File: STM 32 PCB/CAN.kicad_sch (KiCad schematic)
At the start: 6 parts, among them U1 SN65HVD230

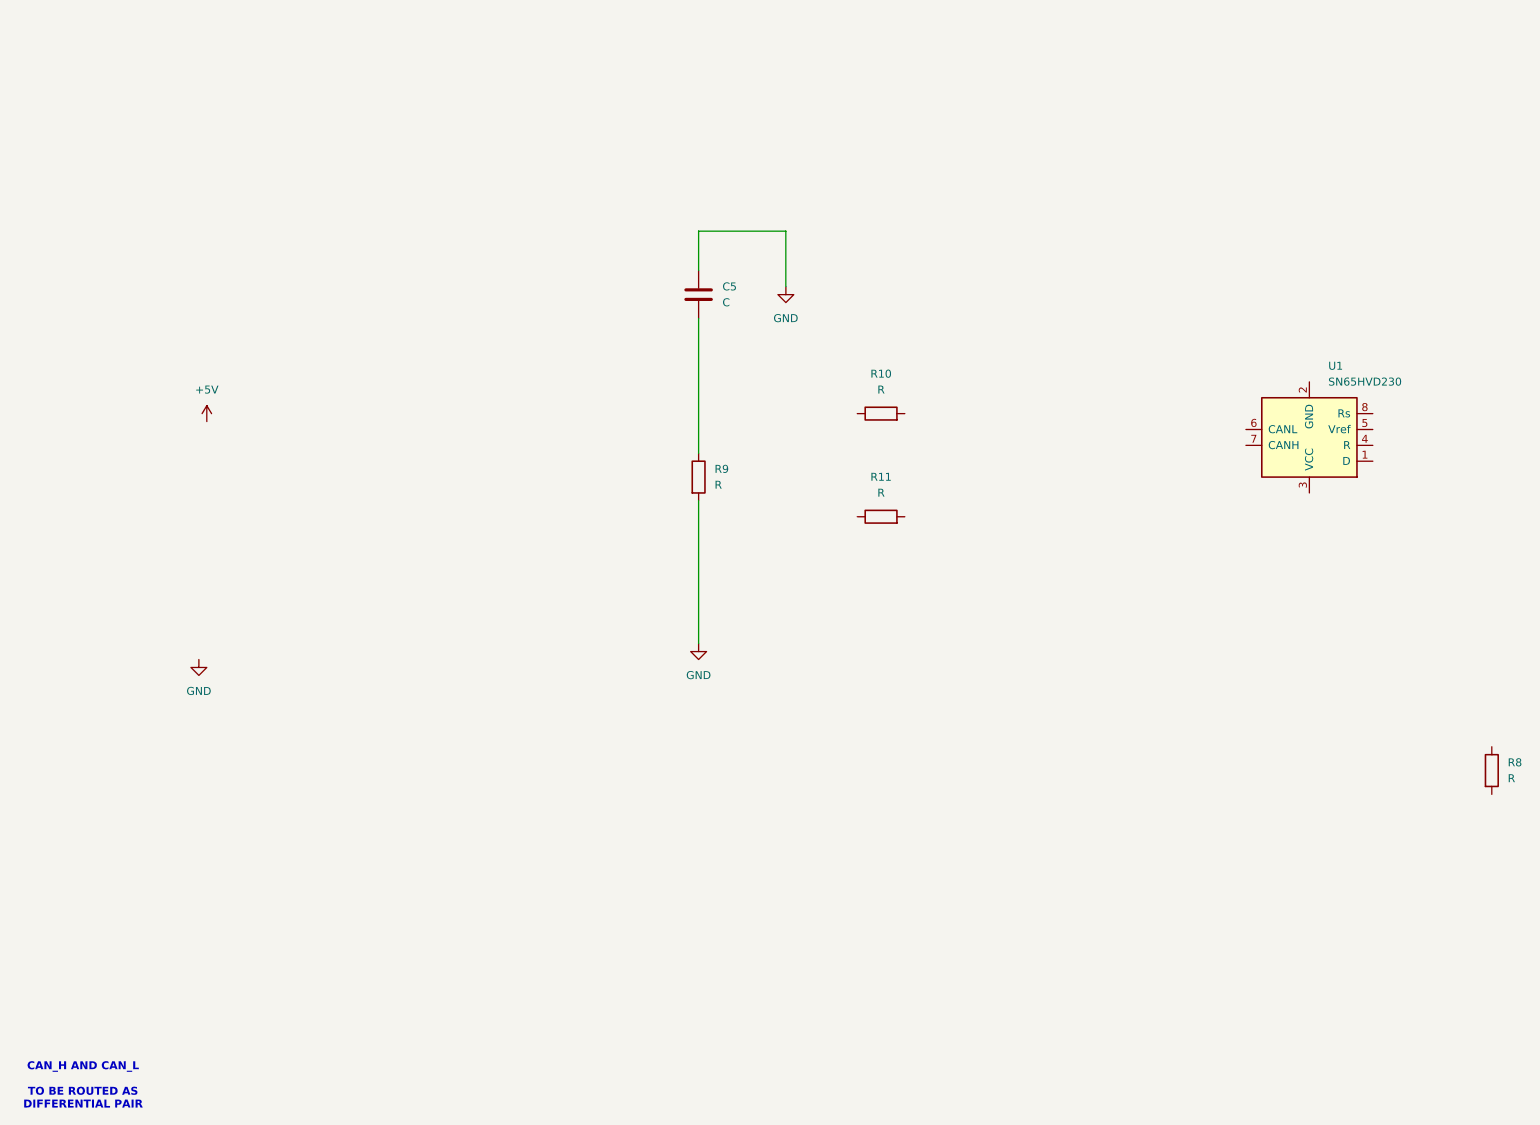
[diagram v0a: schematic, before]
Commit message: 1
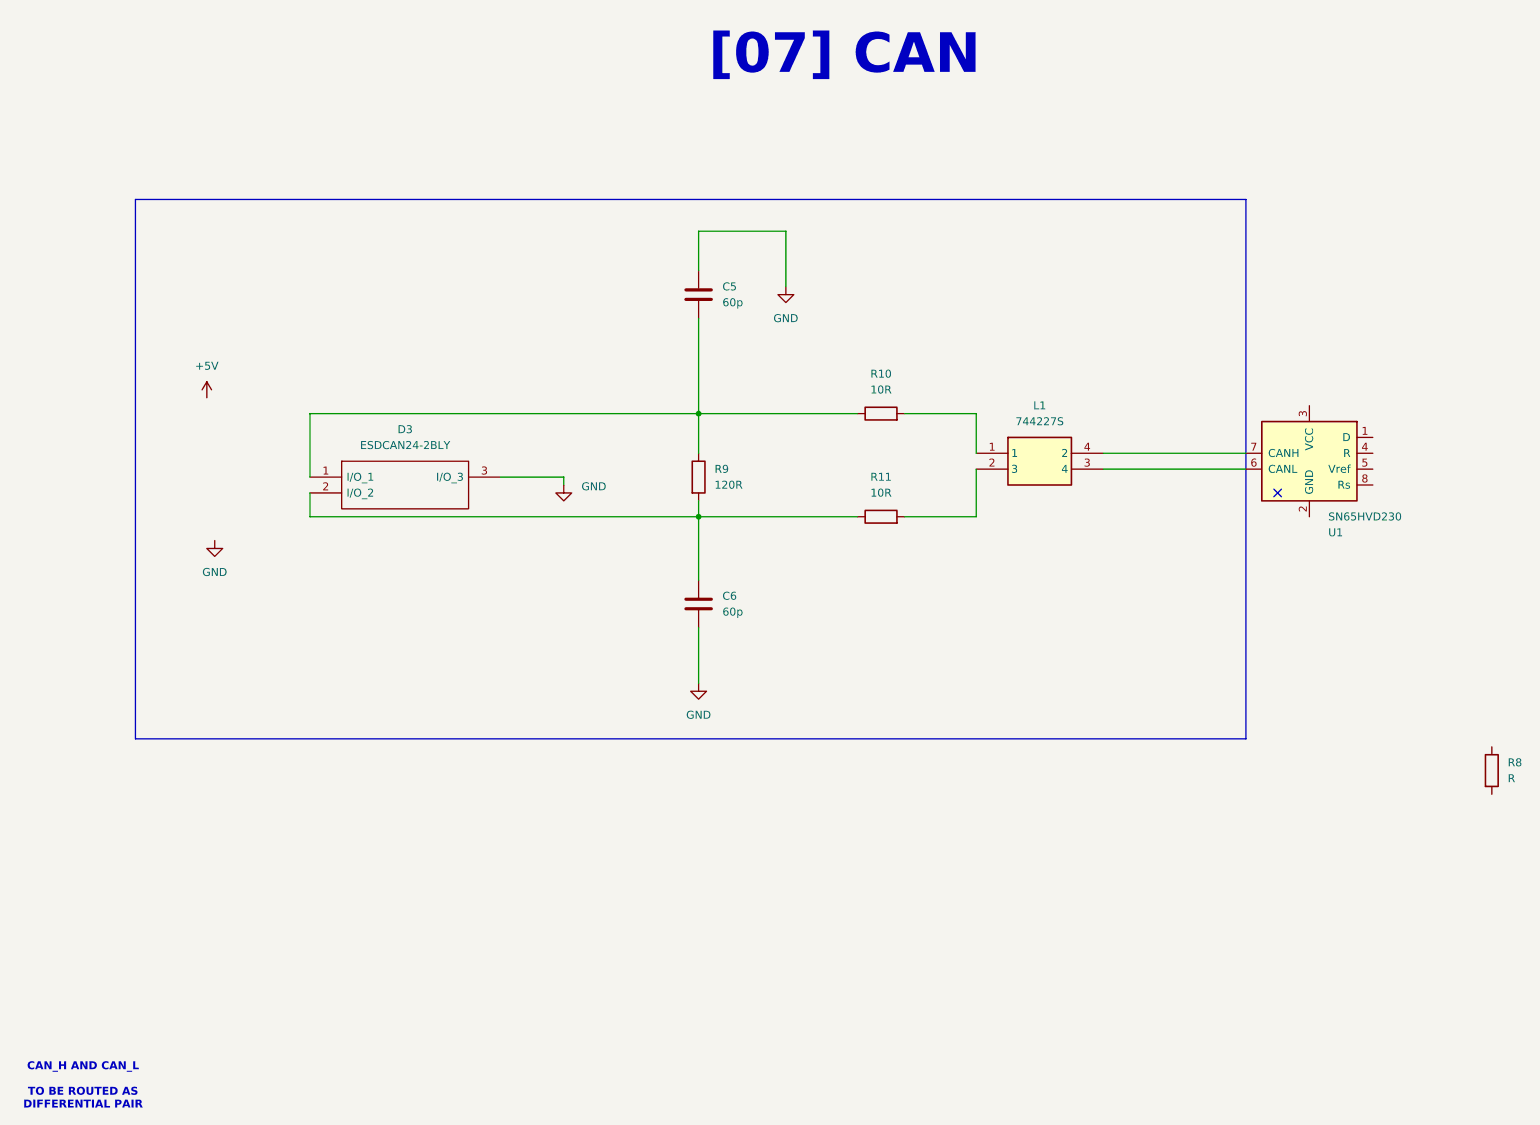
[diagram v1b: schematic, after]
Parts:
- added C6: 60p, symbol Device:C
- added D3: ESDCAN24-2BLY, SOT95P255X125-3N, symbol ESDCAN24-2BLY:ESDCAN24-2BLY
- added L1: 744227S, WE-SL274, symbol 744227S:744227S
- C5: value C -> 60p
- R10, R11: value R -> 10R
- R9: value R -> 120R
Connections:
- net GND: now also C6.2, D3.3 (I/O_3); no longer R9.2
- net at C5.2, R9.1: now also R10.1, D3.1 (I/O_1)
- net at R10.2: now also L1.1
- net at R11.1: now also R9.2, C6.1, D3.2 (I/O_2)
- net at R11.2: now also L1.2 (3)
- net at U1.6 (CANL): now also L1.3 (4)
- net at U1.7 (CANH): now also L1.4 (2)
- no-connect marks 0 -> 1
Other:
- note added: "[07] CAN"
- moved on the sheet: U1
